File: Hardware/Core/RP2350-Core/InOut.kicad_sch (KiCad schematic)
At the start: 20 parts, among them CN10 PR5L4015-5P-C-F, CN11 PR5L4015-5P-C-F, CN7 PR5L4015-5P-C-F, CN8 PR5L4015-5P-C-F, CN9 PR5L4015-5P-C-F, J1 Conn_01x10_Socket, J2 Conn_01x10_Socket, J5 Conn_01x10_Socket, J6 Conn_01x10_Socket, J9 Conn_01x10_Socket, U35 PR5L5015-5P-C-H, U36 PR5L5015-5P-C-H, U37 PR5L5015-5P-C-H, U38 PR5L5015-5P-C-H, U39 PR5L5015-5P-C-H

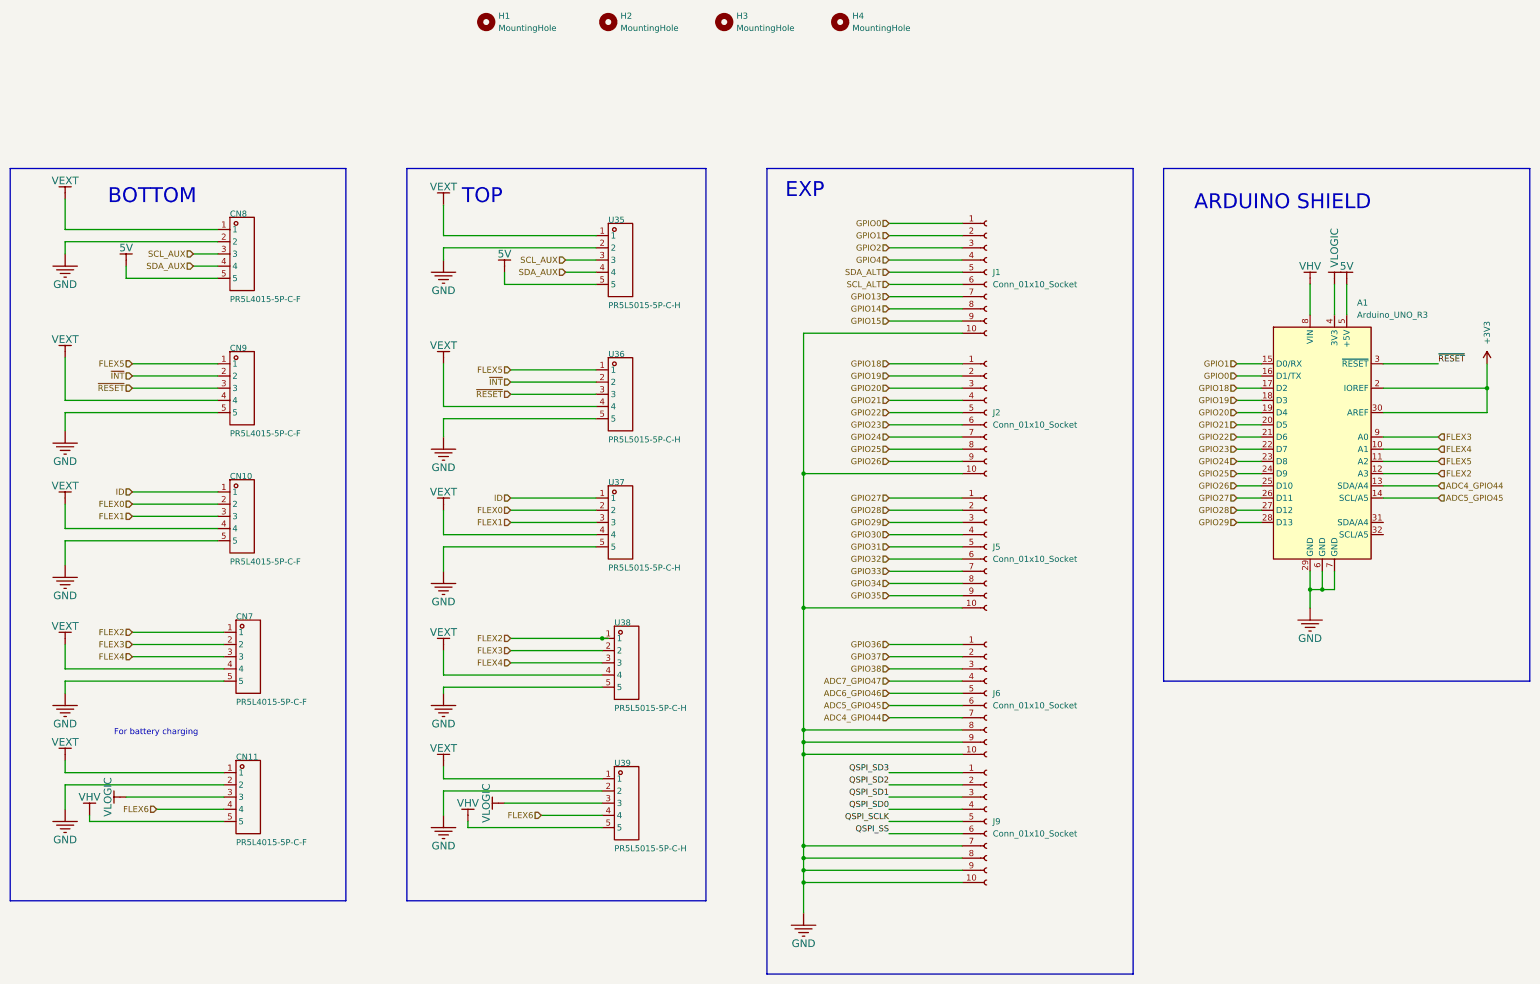
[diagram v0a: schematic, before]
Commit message: Verison RP2350 with arduino header support
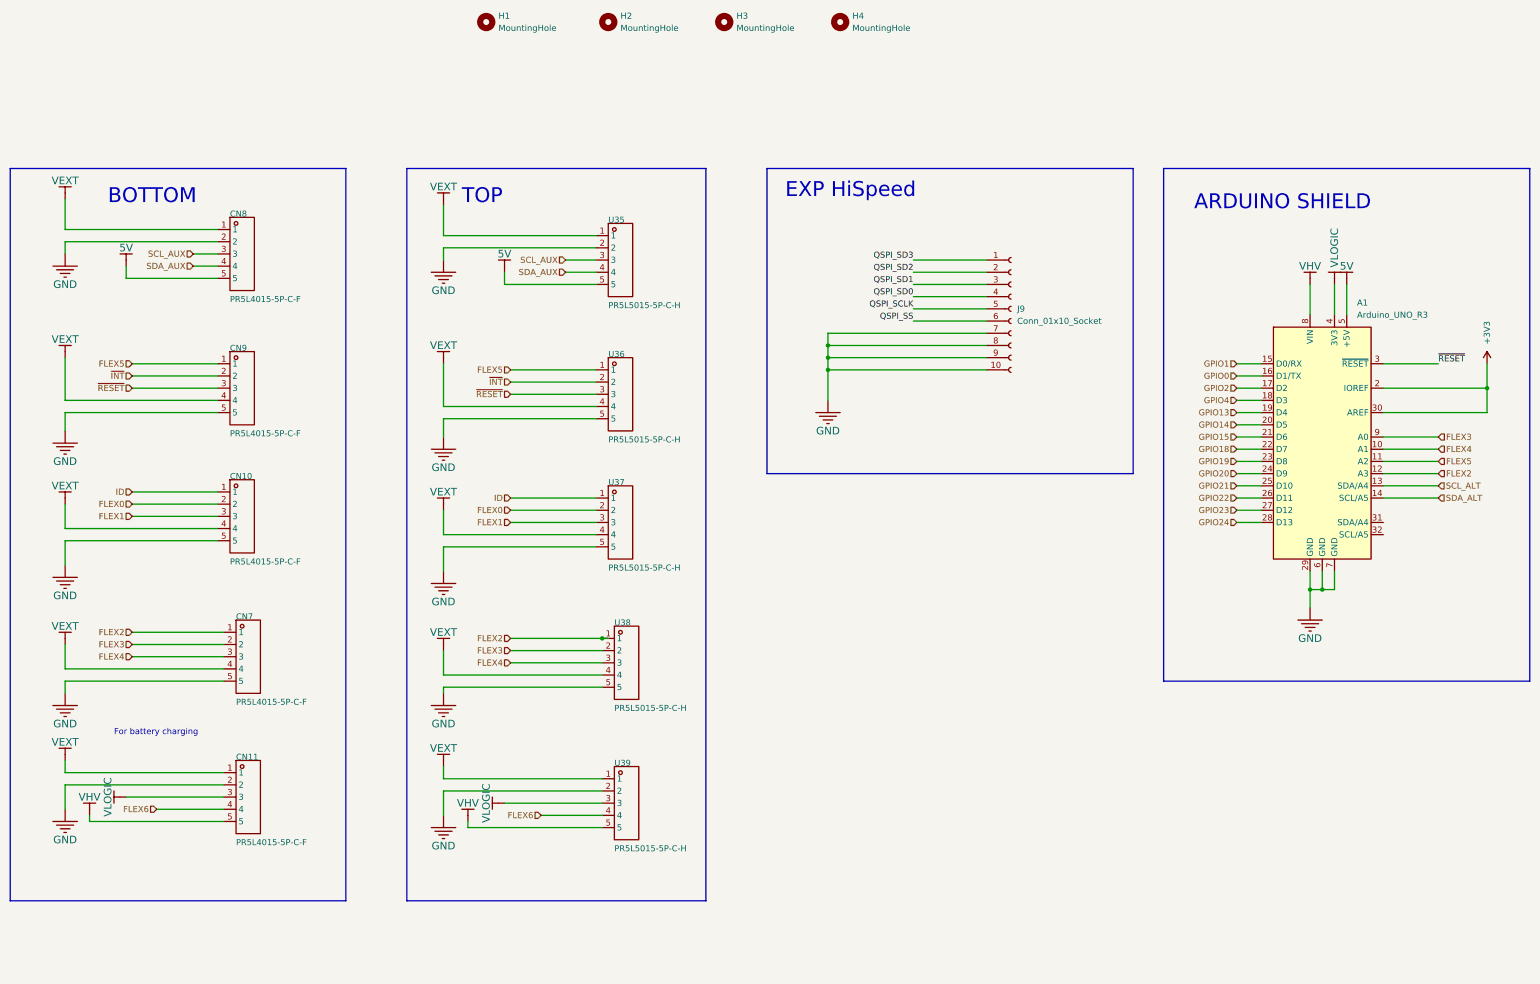
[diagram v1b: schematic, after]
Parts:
- removed J1, J2, J5, J6: Conn_01x10_Socket, Connector_PinHeader_2.54mm:PinHeader_2x10_P2.54mm_Vertical, symbol Connector:Conn_01x10_Socket
- J9: footprint Connector_PinHeader_2.54mm:PinHeader_2x10_P2.54mm_Vertical -> Connector_PinHeader_2.54mm:PinHeader_2x05_P2.54mm_Vertical
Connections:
- net ADC4_GPIO44 is gone; now on net SCL_ALT: A1.13 (SDA/A4)
- net ADC5_GPIO45 is gone; now on net SDA_ALT: A1.14 (SCL/A5)
- net GPIO25 is gone; now on net GPIO20: A1.24 (D9)
- net GPIO26 is gone; now on net GPIO21: A1.25 (D10)
- net GPIO27 is gone; now on net GPIO22: A1.26 (D11)
- net GPIO28 is gone; now on net GPIO23: A1.27 (D12)
- net GPIO29 is gone; now on net GPIO24: A1.28 (D13)
- net GPIO13: now also A1.19 (D4)
- net GPIO14: now also A1.20 (D5)
- net GPIO15: now also A1.21 (D6)
- net GPIO18: now also A1.22 (D7); no longer A1.17 (D2)
- net GPIO19: now also A1.23 (D8); no longer A1.18 (D3)
- net GPIO2: now also A1.17 (D2)
- net GPIO20: no longer A1.19 (D4)
- net GPIO21: no longer A1.20 (D5)
- net GPIO22: no longer A1.21 (D6)
- net GPIO23: no longer A1.22 (D7)
- net GPIO24: no longer A1.23 (D8)
- net GPIO4: now also A1.18 (D3)
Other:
- note added: "EXP HiSpeed"
- note removed: "EXP"
- moved on the sheet: J9

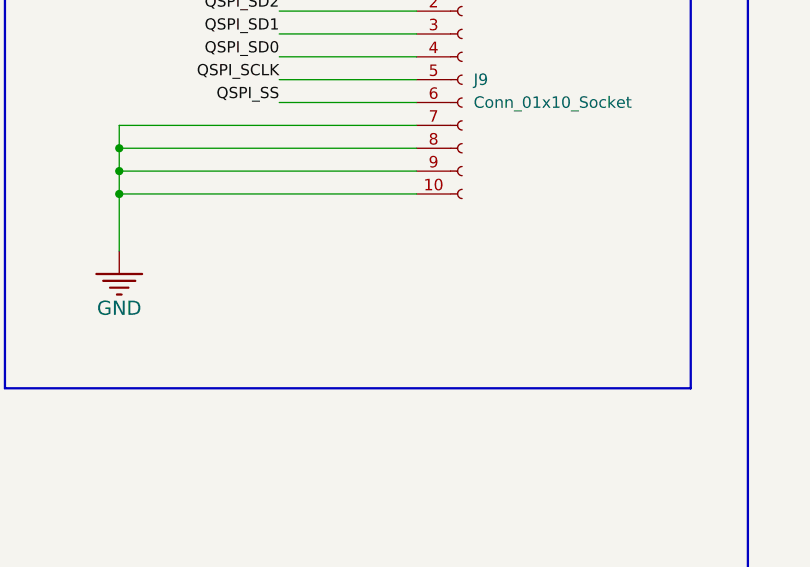
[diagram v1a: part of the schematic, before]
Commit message: Connectors connection improvements
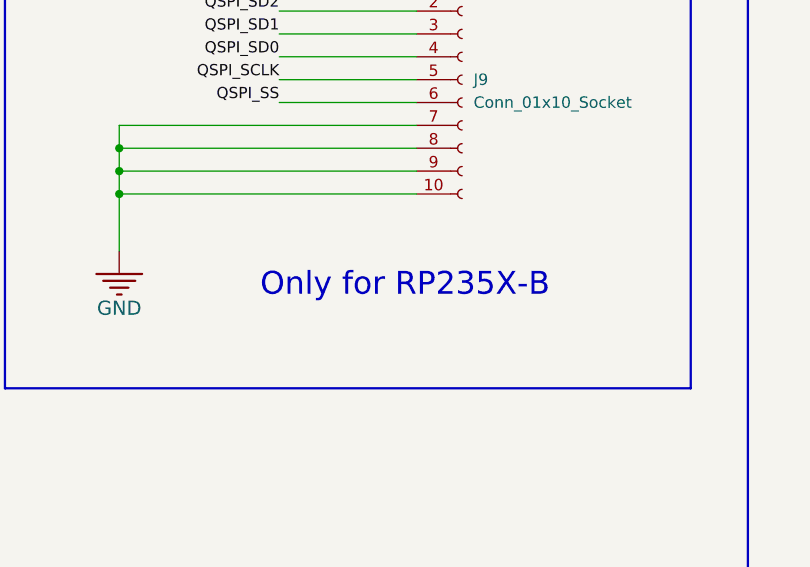
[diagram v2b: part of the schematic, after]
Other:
- note added: "Only for RP235X-B"
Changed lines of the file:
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@@
+		)
+	)
+	(text "Only for RP235X-B"
+		(exclude_from_sim no)
+		(at 256.54 111.76 0)
+		(effects
+			(font
+				(size 2.54 2.54)
+			)
 		)
 	)
